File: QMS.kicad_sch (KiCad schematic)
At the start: 6 parts, among them J1 Screw_Terminal_01x02, J2 PINHD_1x5_Male, J3 PINHD_1x3_Male, U1 ESP-12E, U2 AMS1117-3.3

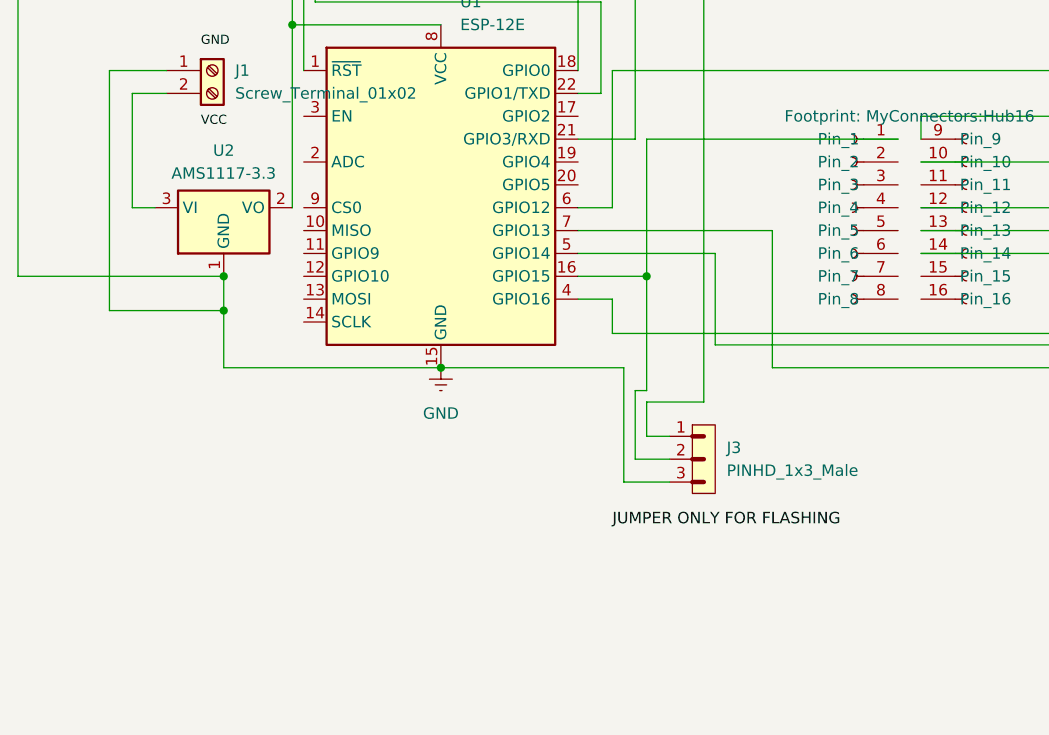
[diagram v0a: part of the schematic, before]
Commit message: completed
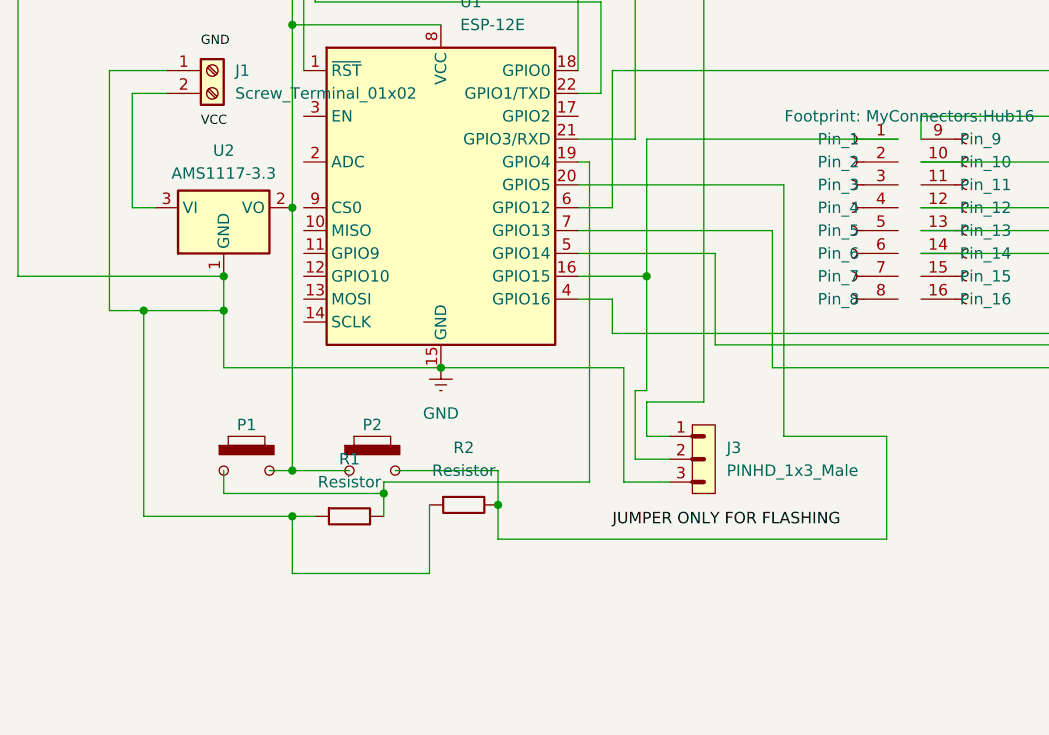
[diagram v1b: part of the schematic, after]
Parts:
- added P1, P2: ~, Button_Switch_THT:SW_PUSH-12mm, symbol PCM_Nuova-Elettronica-Switches:Push_Button
- added R1, R2: Resistor, Resistor_THT:R_Axial_DIN0207_L6.3mm_D2.5mm_P7.62mm_Horizontal, symbol PCM_SL_Resistors:Resistor
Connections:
- net GND: now also R1.1, R2.1
- net VCC 3.3v: now also P1.2, P2.1
- net at U1.19 (GPIO4): now also P1.1, R1.2
- net at U1.20 (GPIO5): now also P2.2, R2.2
